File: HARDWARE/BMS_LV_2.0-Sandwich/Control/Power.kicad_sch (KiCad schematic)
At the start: 25 parts, among them IC1 TAR5S33UTE85LF, IC4 TPS54202HDDCR

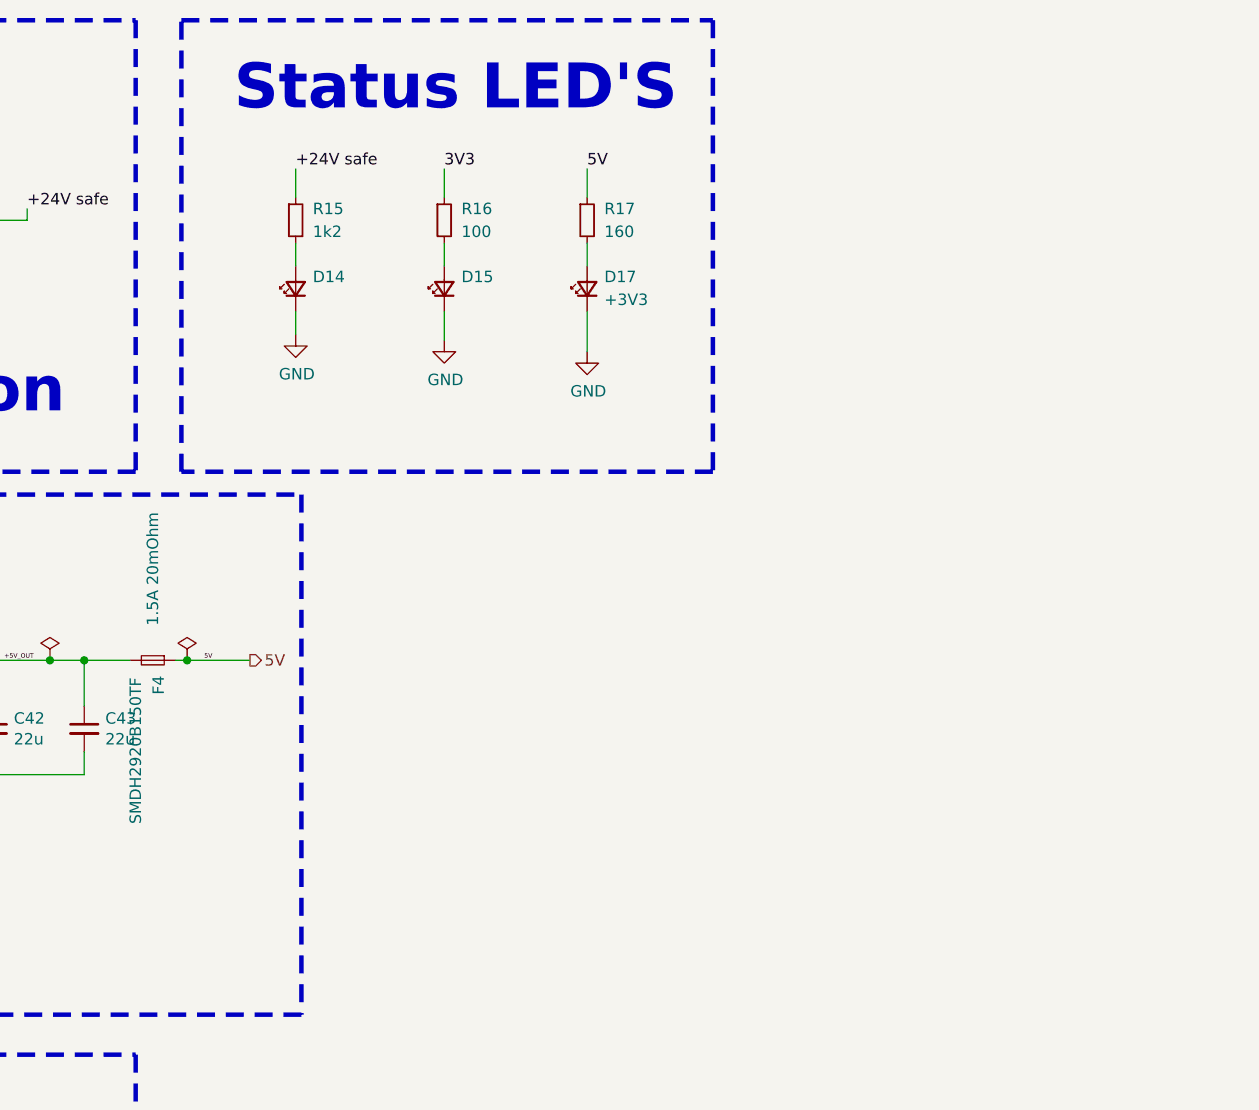
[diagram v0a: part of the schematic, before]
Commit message: Ulozono silkscreena
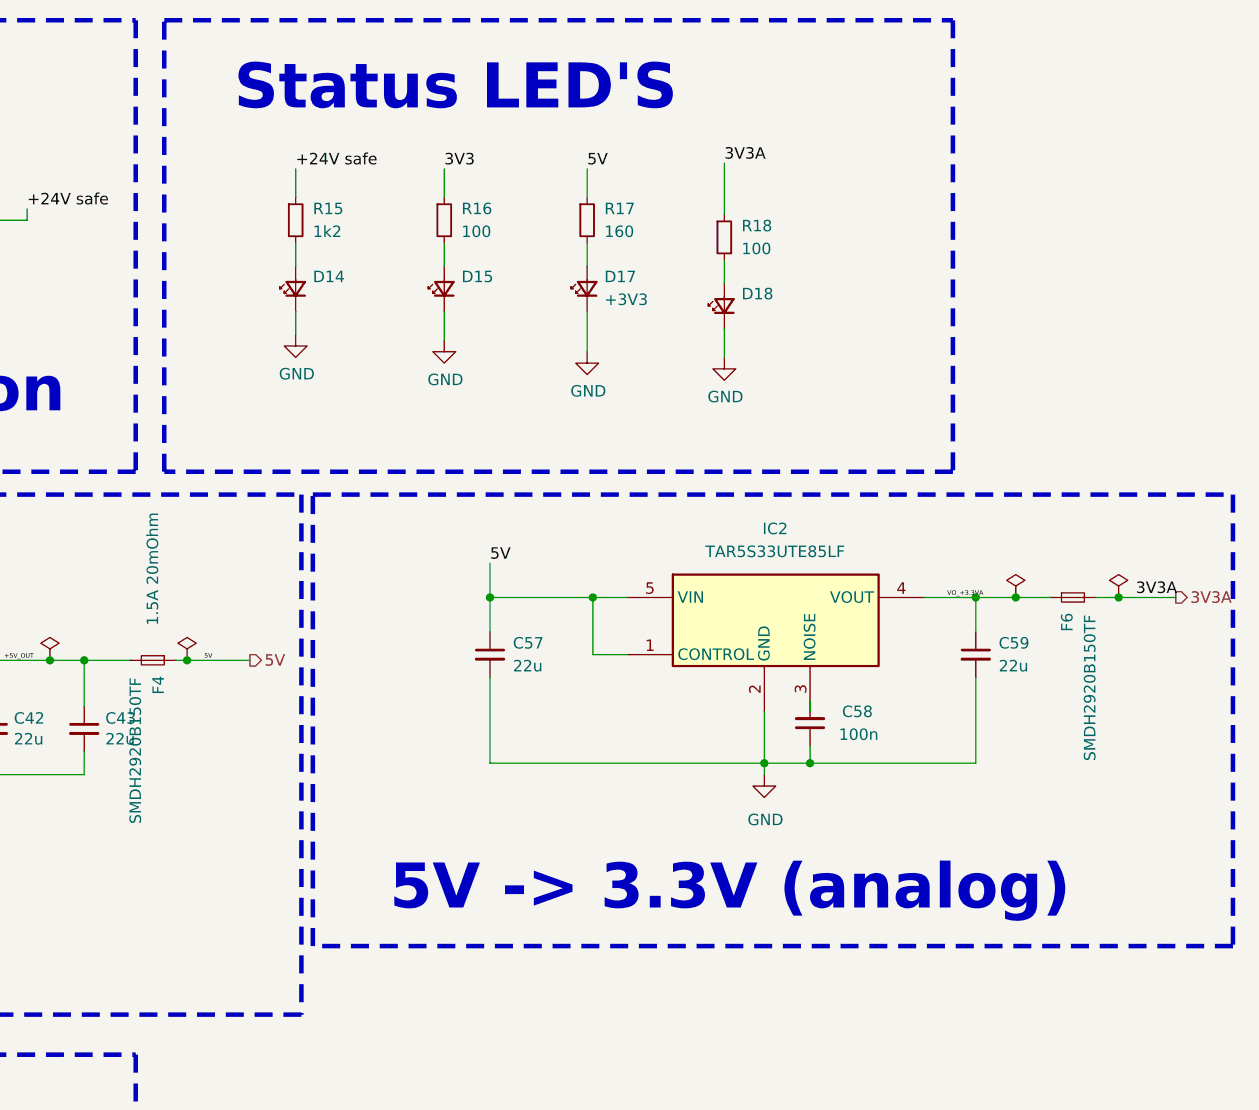
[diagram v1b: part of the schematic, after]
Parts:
- added C57, C59: 22u, Capacitor_SMD:C_0805_2012Metric_Pad1.18x1.45mm_HandSolder, symbol Device:C_Small
- added C58: 100n, Capacitor_SMD:C_0603_1608Metric, symbol Device:C_Small
- added D18: ~, LED_SMD:LED_0603_1608Metric_Pad1.05x0.95mm_HandSolder, symbol Device:LED_Small
- added F6: SMDH2920B150TF, Fuse:Fuse_2920_7451Metric_Pad2.10x5.45mm_HandSolder, symbol Device:Fuse_Small
- added IC2: TAR5S33UTE85LF, Footprint:SOTFL65P210X75-5N, symbol TAR5S33UTE85LF:TAR5S33UTE85LF
- added R18: 100, Resistor_SMD:R_0603_1608Metric_Pad0.98x0.95mm_HandSolder, symbol Device:R_Small
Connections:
- net 5V: now also C57.1, IC2.1 (CONTROL), IC2.5 (VIN)
- net GND: now also C57.2, C58.1, C59.2, D18.1 (K), IC2.2 (GND)
- new net: C58.2, IC2.3 (NOISE)
- new net: D18.2 (A), R18.2
- new net 3V3A: F6.2, R18.1
- new net VO_+3.3VA: C59.1, F6.1, IC2.4 (VOUT)
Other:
- note added: "5V -> 3.3V (analog)"
